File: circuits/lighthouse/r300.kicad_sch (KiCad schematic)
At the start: 18 parts, among them Q3 2N7002K, U1 R300, U6 AMS1117-3.3

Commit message: Rewamped the pcb
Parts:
- BZ1: footprint Buzzer_Beeper:Buzzer_12x9.5RM7.6 -> Buzzer_Beeper:MagneticBuzzer_PUI_AT-0927-TT-6-R
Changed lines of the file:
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@@
 			)
 		)
-		(property "Footprint" "Buzzer_Beeper:Buzzer_12x9.5RM7.6"
+		(property "Footprint" "Buzzer_Beeper:MagneticBuzzer_PUI_AT-0927-TT-6-R"
 			(at 97.79 123.825 90)
 			(effects

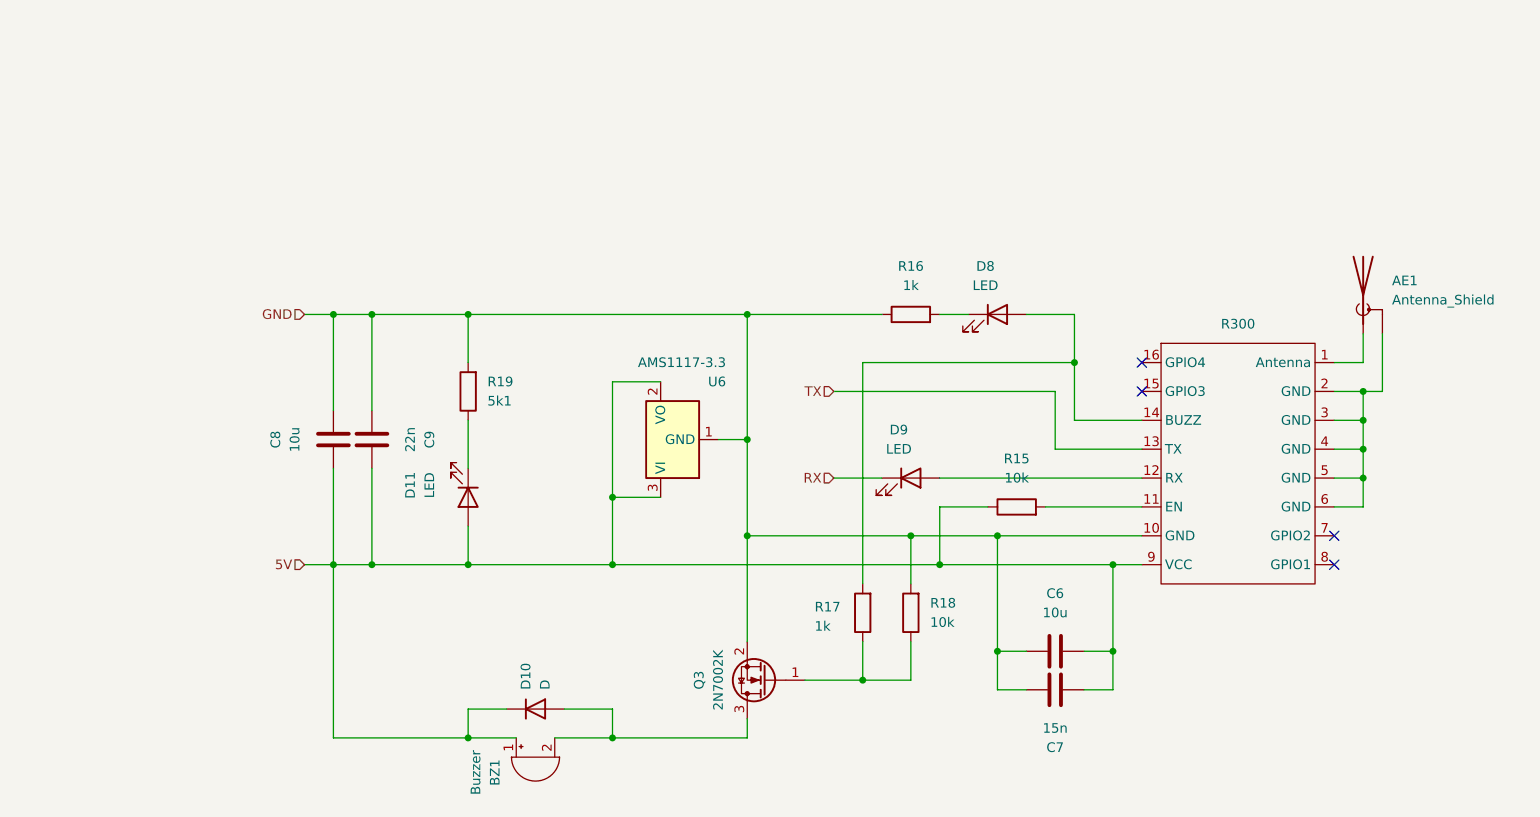
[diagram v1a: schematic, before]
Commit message: Cleaned up schematics
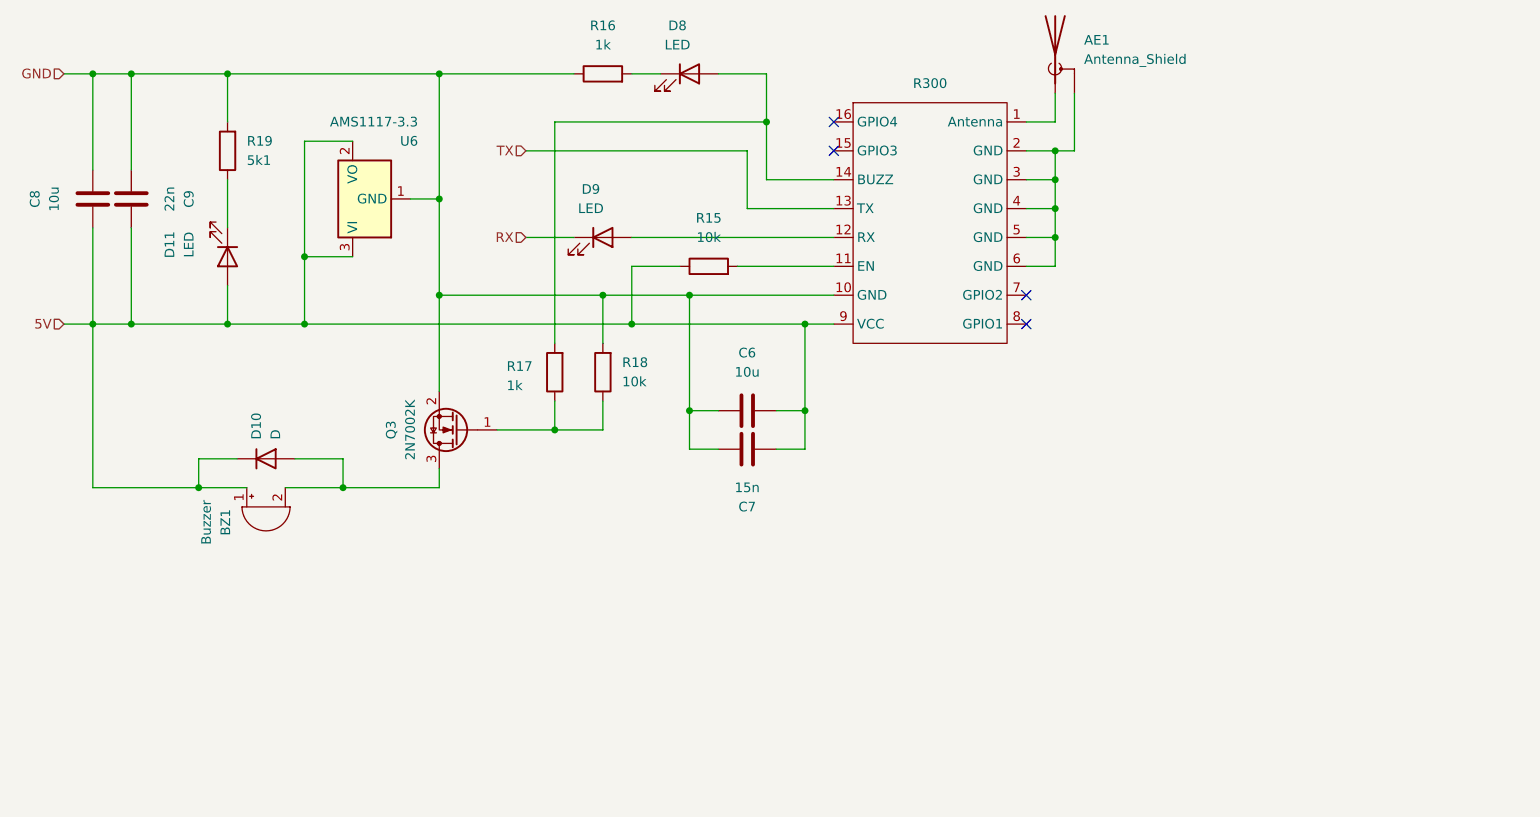
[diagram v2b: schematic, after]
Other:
- moved on the sheet: AE1, BZ1, C6, C7, C8, C9, D10, D11, D8, D9, Q3, R15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
